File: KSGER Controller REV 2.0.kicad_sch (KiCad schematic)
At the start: 51 parts, among them J1 24 VDC, J2 IRON_IN, J4 BATT, J5 SWD, Q1 IRF7416, Q2 S8050, SW1 ENCODER, U1 STM32F103C8Tx, U2 AMS1117-3.3, U3 SGM8551, U4 24LC08, U6 L78L08_SOT89, U7 SSD1106, Y1 32.768MHz

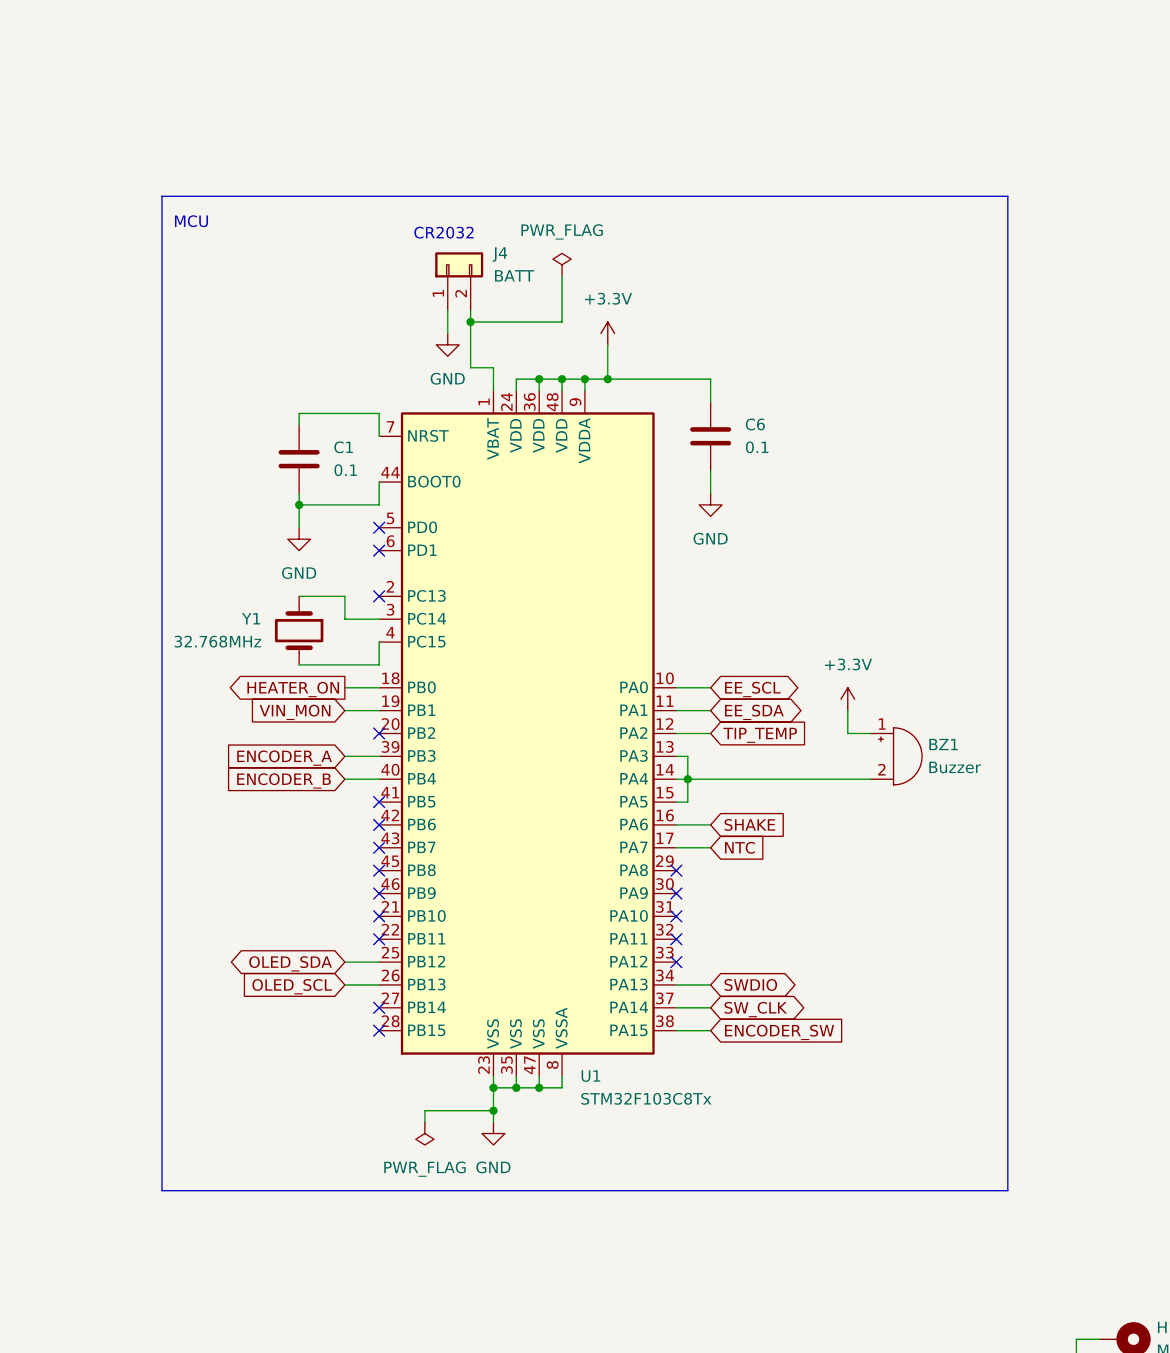
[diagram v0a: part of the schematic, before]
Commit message: Working on trace redesign for v2
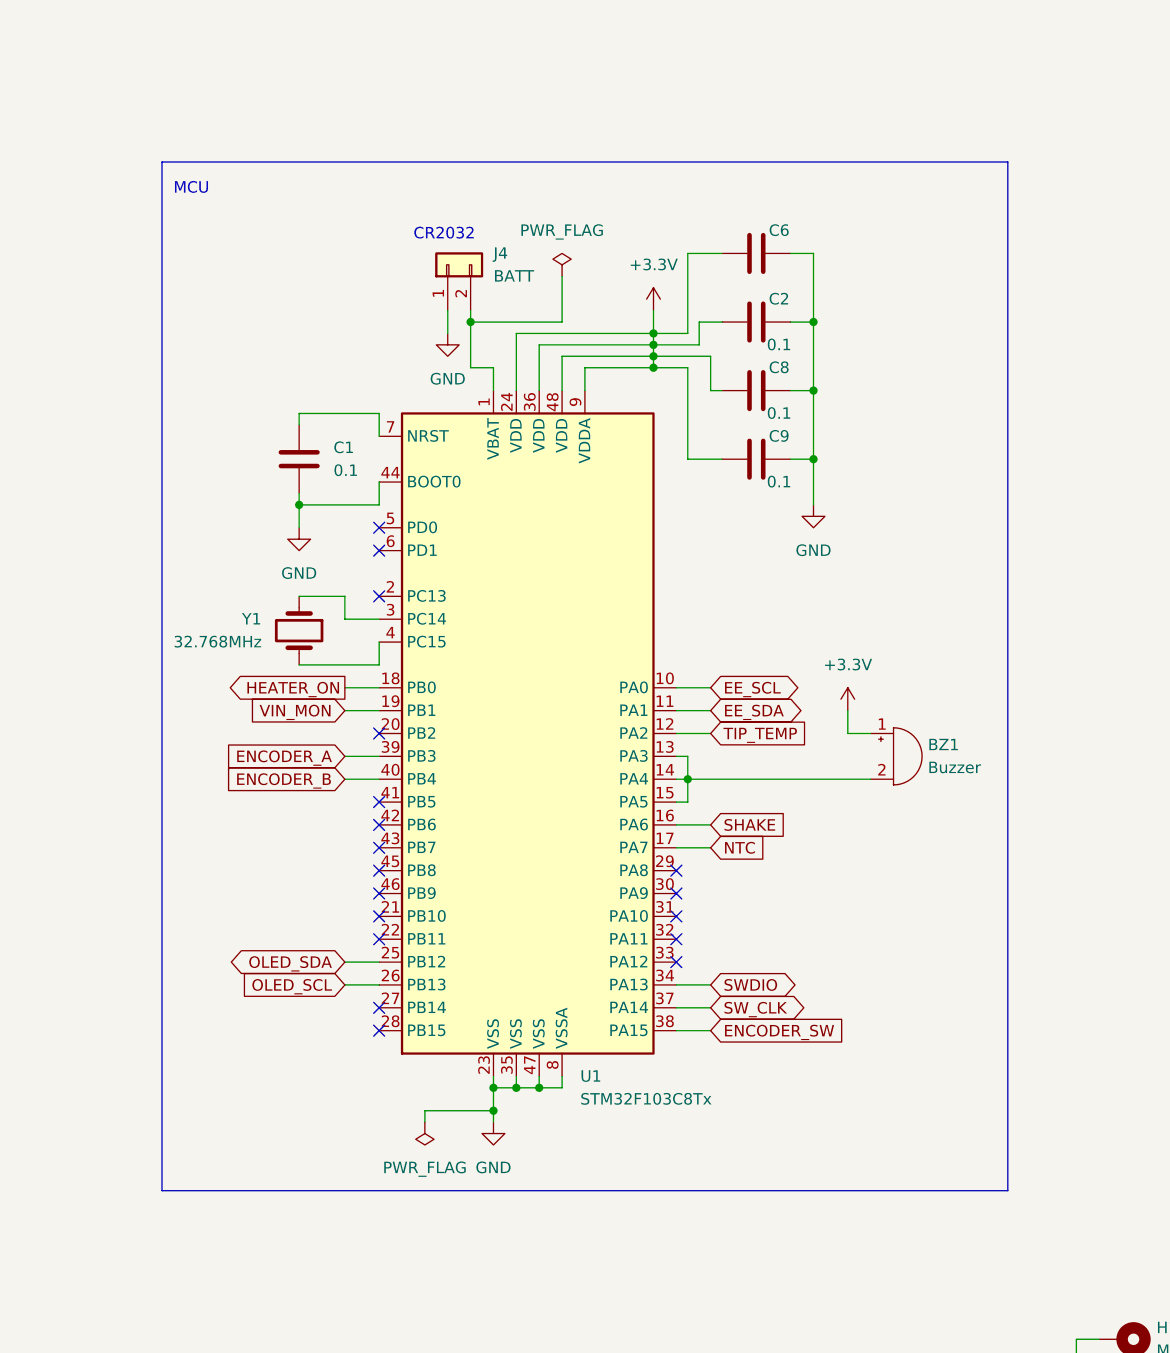
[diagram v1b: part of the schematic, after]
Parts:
- added C2, C8, C9: 0.1, Capacitor_SMD:C_0201_0603Metric, symbol Device:C
- C6: value 0.1 -> (none); footprint Capacitor_SMD:C_0805_2012Metric -> (none); JCLPCB Part # C49678 -> C14663
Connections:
- net +3V3: now also C2.1, C8.1, C9.1
- net GND: now also C2.2, C8.2, C9.2
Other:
- moved on the sheet: C6
